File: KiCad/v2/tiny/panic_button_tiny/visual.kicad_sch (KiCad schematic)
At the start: 1 part, among them U4 TPS61022

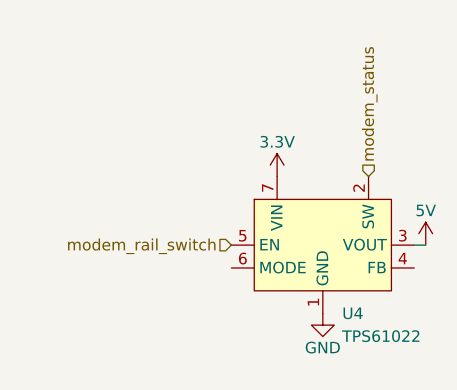
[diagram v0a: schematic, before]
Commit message: [UPDATE] some connections in the schematic
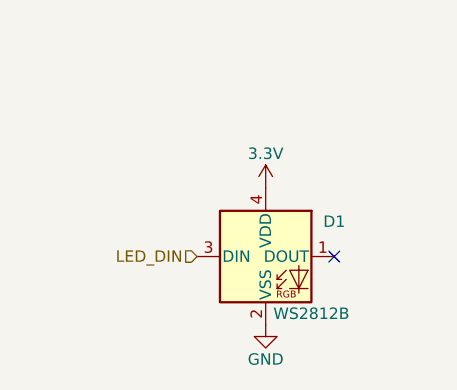
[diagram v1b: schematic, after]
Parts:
- removed U4: TPS61022, Package_DFN_QFN:Texas_RWU0007A_VQFN-7_2x2mm_P0.5mm, symbol Converter_DCDC:TPS61022
- added D1: WS2812B, PCM_SparkFun-LED:WS2812_2020, symbol PCM_SparkFun-LED:WS2812B_2020
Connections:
- net 3.3V: now also D1.4 (VDD)
- net GND: now also D1.2 (VSS)
- new net LED_DIN: D1.3 (DIN)
- no-connect marks 0 -> 1
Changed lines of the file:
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@@
 	(generator_version "10.0")
 	(paper "A4")
-	(wire
-		(pts
-			(xy 62.23 30.48) (xy 60.96 30.48)
-		)
-		(stroke
-			(width 0)
-			(type default)
-		)
-	)
-	(hierarchical_label "modem_status"
+	(no_connect
+		(at 52.07 31.75)
+	)
+	(hierarchical_label "LED_DIN"
 		(shape input)
-		(at 55.88 22.86 90)
+		(at 36.83 31.75 180)
 		(effects
 			(font
 				(size 1.27 1.27)
 			)
-			(justify left)
-		)
-	)
-	(hierarchical_label "modem_rail_switch"
-		(shape input)
-		(at 40.64 30.48 180)
-		(effects
-			(font
-				(size 1.27 1.27)
-			)
 			(justify right)
 		)
@@
 	(symbol
 		(lib_id "PCM_SparkFun-PowerSymbol:3.3V")
-		(at 45.72 22.86 0)
+		(at 44.45 24.13 0)
 		(unit 1)
 		(body_style 1)
@@
 		(dnp no)
 		(fields_autoplaced yes)
-		(property "Reference" "#PWR048"
-			(at 45.72 26.67 0)
+		(property "Reference" "#PWR064"
+			(at 44.45 27.94 0)
 			(hide yes)
 			(show_name no)
@@
 		)
 		(property "Value" "3.3V"
-			(at 45.72 19.05 0)
+			(at 44.45 20.32 0)
 			(show_name no)
 			(do_not_autoplace yes)
@@
 		)
 		(property "Footprint" ""
-			(at 45.72 22.86 0)
+			(at 44.45 24.13 0)
 			(hide yes)
 			(show_name no)
@@
 		)
 		(property "Datasheet" ""
-			(at 45.72 22.86 0)
+			(at 44.45 24.13 0)
 			(hide yes)
 			(show_name no)
@@
 		)
 		(property "Description" "Power symbol creates a global label with name \"3.3V\""
-			(at 45.72 29.21 0)
+			(at 44.45 30.48 0)
 			(hide yes)
 			(show_name no)
@@
 		(instances
 			(project "panic_button_tiny"
-				(path "/c4eb92e9-b42f-4db0-b1d9-0ef70f7ca601/5fcd7ab2-c492-450d-9345-ebba8273bb1f"
-					(reference "#PWR048")
+				(path "/c4eb92e9-b42f-4db0-b1d9-0ef70f7ca601/a5c86ac0-c7fd-4e96-b586-e8495a668fc4"
+					(reference "#PWR064")
 					(unit 1)
 				)
@@
 	)
 	(symbol
-		(lib_id "PCM_SparkFun-PowerSymbol:5V")
-		(at 62.23 30.48 0)
+		(lib_id "PCM_SparkFun-PowerSymbol:GND")
+		(at 44.45 39.37 0)
 		(unit 1)
 		(body_style 1)
@@
 		(dnp no)
 		(fields_autoplaced yes)
-		(property "Reference" "#PWR050"
-			(at 62.23 34.29 0)
-			(hide yes)
-			(show_name no)
-			(do_not_autoplace no)
-			(effects
-				(font
-					(size 1.27 1.27)
-				)
-			)
-		)
-		(property "Value" "5V"
-			(at 62.23 26.67 0)
+		(property "Reference" "#PWR065"
+			(at 44.45 45.72 0)
+			(hide yes)
+			(show_name no)
+			(do_not_autoplace no)
+			(effects
+				(font
+					(size 1.27 1.27)
+				)
+			)
+		)
+		(property "Value" "GND"
+			(at 44.45 43.18 0)
 			(show_name no)
 			(do_not_autoplace yes)
@@
 		)
 		(property "Footprint" ""
-			(at 62.23 30.48 0)
+			(at 44.45 39.37 0)
 			(hide yes)
 			(show_name no)
@@
 		)
 		(property "Datasheet" ""
-			(at 62.23 30.48 0)
-			(hide yes)
-			(show_name no)
-			(do_not_autoplace no)
-			(effects
-				(font
-					(size 1.27 1.27)
-				)
-			)
-		)
-		(property "Description" "Power symbol creates a global label with name \"5V\""
-			(at 62.23 36.83 0)
+			(at 44.45 39.37 0)
+			(hide yes)
+			(show_name no)
+			(do_not_autoplace no)
+			(effects
+				(font
+					(size 1.27 1.27)
+				)
+			)
+		)
+		(property "Description" "Power symbol creates a global label with name \"GND\" , ground"
+			(at 44.45 48.26 0)
 			(hide yes)
 			(show_name no)
@@
 		(instances
 			(project "panic_button_tiny"
-				(path "/c4eb92e9-b42f-4db0-b1d9-0ef70f7ca601/5fcd7ab2-c492-450d-9345-ebba8273bb1f"
-					(reference "#PWR050")
+				(path "/c4eb92e9-b42f-4db0-b1d9-0ef70f7ca601/a5c86ac0-c7fd-4e96-b586-e8495a668fc4"
+					(reference "#PWR065")
 					(unit 1)
 				)
@@
 	)
 	(symbol
-		(lib_id "Converter_DCDC:TPS61022")
-		(at 50.8 30.48 0)
+		(lib_id "PCM_SparkFun-LED:WS2812B_2020")
+		(at 44.45 31.75 0)
 		(unit 1)
 		(body_style 1)
@@
 		(dnp no)
 		(fields_autoplaced yes)
-		(property "Reference" "U4"
-			(at 52.9433 38.1 0)
-			(show_name no)
-			(do_not_autoplace no)
-			(effects
-				(font
-					(size 1.27 1.27)
-				)
-				(justify left)
-			)
-		)
-		(property "Value" "TPS61022"
-			(at 52.9433 40.64 0)
-			(show_name no)
-			(do_not_autoplace no)
-			(effects
-				(font
-					(size 1.27 1.27)
-				)
-				(justify left)
-			)
-		)
-		(property "Footprint" "Package_DFN_QFN:Texas_RWU0007A_VQFN-7_2x2mm_P0.5mm"
-			(at 50.8 53.34 0)
-			(hide yes)
-			(show_name no)
-			(do_not_autoplace no)
-			(effects
-				(font
-					(size 1.27 1.27)
-				)
-			)
-		)
-		(property "Datasheet" "https://www.ti.com/lit/ds/symlink/tps61022.pdf"
-			(at 50.8 55.88 0)
-			(hide yes)
-			(show_name no)
-			(do_not_autoplace no)
-			(effects
-				(font
-					(size 1.27 1.27)
-				)
-			)
-		)
-		(property "Description" "8A Boost Converter, 0.5-5.5 V input, 2.2-5.5V output, Texas RWU0007A VQFN-7"
-			(at 50.8 30.48 0)
-			(hide yes)
-			(show_name no)
-			(do_not_autoplace no)
-			(effects
-				(font
-					(size 1.27 1.27)
-				)
-			)
+		(property "Reference" "D1"
+			(at 52.07 27.8698 0)
+			(show_name no)
+			(do_not_autoplace no)
+			(effects
+				(font
+					(size 1.27 1.27)
+				)
+			)
+		)
+		(property "Value" "WS2812B"
+			(at 49.53 38.1 0)
+			(show_name no)
+			(do_not_autoplace yes)
+			(effects
+				(font
+					(size 1.27 1.27)
+				)
+			)
+		)
+		(property "Footprint" "PCM_SparkFun-LED:WS2812_2020"
+			(at 44.45 41.91 0)
+			(hide yes)
+			(show_name no)
+			(do_not_autoplace no)
+			(effects
+				(font
+					(size 1.27 1.27)
+				)
+			)
+		)
+		(property "Datasheet" "https://cdn.sparkfun.com/assets/e/1/0/f/b/WS2812C-2020_V1.2_EN_19112716191654.pdf"
+			(at 44.45 46.99 0)
+			(hide yes)
+			(show_name no)
+			(do_not_autoplace no)
+			(effects
+				(font
+					(size 1.27 1.27)
+				)
+			)
+		)
+		(property "Description" "RGB LED with integrated controller"
+			(at 44.45 49.53 0)
+			(hide yes)
+			(show_name no)
+			(do_not_autoplace no)
+			(effects
+				(font
+					(size 1.27 1.27)
+				)
+			)
+		)
+		(property "PROD_ID" "DIO-15591"
+			(at 44.45 44.45 0)
+			(hide yes)
+			(show_name no)
+			(do_not_autoplace no)
+			(effects
+				(font
+					(size 1.27 1.27)
+				)
+			)
+		)
+		(pin "4"
+		)
+		(pin "3"
 		)
 		(pin "2"
 		)
-		(pin "4"
-		)
-		(pin "7"
-		)
-		(pin "6"
-		)
 		(pin "1"
-		)
-		(pin "3"
-		)
-		(pin "5"
 		)
 		(instances
 			(project "panic_button_tiny"
-				(path "/c4eb92e9-b42f-4db0-b1d9-0ef70f7ca601/5fcd7ab2-c492-450d-9345-ebba8273bb1f"
-					(reference "U4")
+				(path "/c4eb92e9-b42f-4db0-b1d9-0ef70f7ca601/a5c86ac0-c7fd-4e96-b586-e8495a668fc4"
+					(reference "D1")
 					(unit 1)
 				)
-			)
-		)
-	)
-	(symbol
-		(lib_id "PCM_SparkFun-PowerSymbol:GND")
-		(at 50.8 38.1 0)
-		(unit 1)
-		(body_style 1)
-		(exclude_from_sim no)
-		(in_bom yes)
-		(on_board yes)
-		(in_pos_files yes)
-		(dnp no)
-		(fields_autoplaced yes)
-		(property "Reference" "#PWR049"
-			(at 50.8 44.45 0)
-			(hide yes)
-			(show_name no)
-			(do_not_autoplace no)
-			(effects
-				(font
-					(size 1.27 1.27)
-				)
-			)
-		)
-		(property "Value" "GND"
-			(at 50.8 41.91 0)
-			(show_name no)
-			(do_not_autoplace yes)
-			(effects
-				(font
-					(size 1.27 1.27)
-				)
-			)
-		)
-		(property "Footprint" ""
-			(at 50.8 38.1 0)
-			(hide yes)
-			(show_name no)
-			(do_not_autoplace no)
-			(effects
-				(font
-					(size 1.27 1.27)
-				)
-			)
-		)
-		(property "Datasheet" ""
-			(at 50.8 38.1 0)
-			(hide yes)
-			(show_name no)
-			(do_not_autoplace no)
-			(effects
-				(font
-					(size 1.27 1.27)
-				)
-			)
-		)
-		(property "Description" "Power symbol creates a global label with name \"GND\" , ground"
-			(at 50.8 46.99 0)
-			(hide yes)
-			(show_name no)
-			(do_not_autoplace no)
-			(effects
-				(font
-					(size 1.27 1.27)
-				)
-			)
-		)
-		(pin "1"
-		)
-		(instances
-			(project "panic_button_tiny"
-				(path "/c4eb92e9-b42f-4db0-b1d9-0ef70f7ca601/5fcd7ab2-c492-450d-9345-ebba8273bb1f"
-					(reference "#PWR049")
-					(unit 1)
-				)
